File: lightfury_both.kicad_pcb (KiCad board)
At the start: 6 copper layers, 168.2 x 217.8 mm, 184 parts, among them U1 TLV61070ADBV, U1_2 TLV61070ADBV, U2 SN74LV1T126DBVR, U2_2 SN74LV1T126DBVR

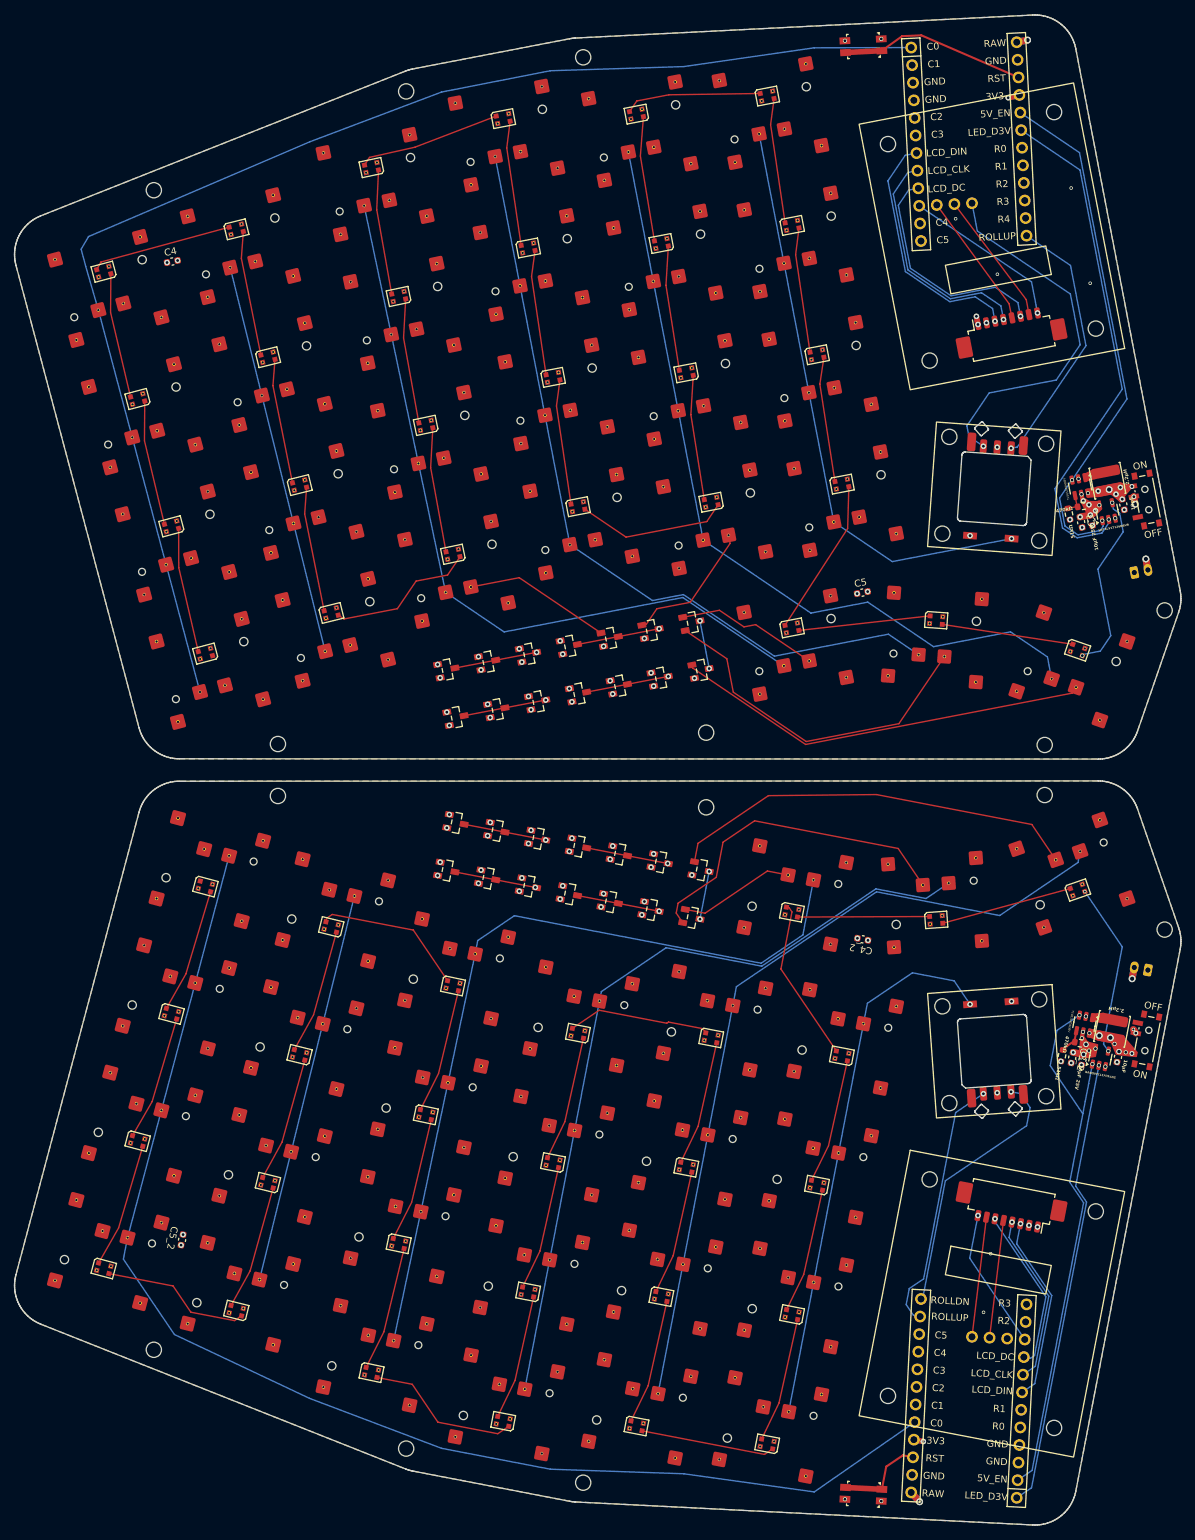
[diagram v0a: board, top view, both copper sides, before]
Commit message: Cleanup
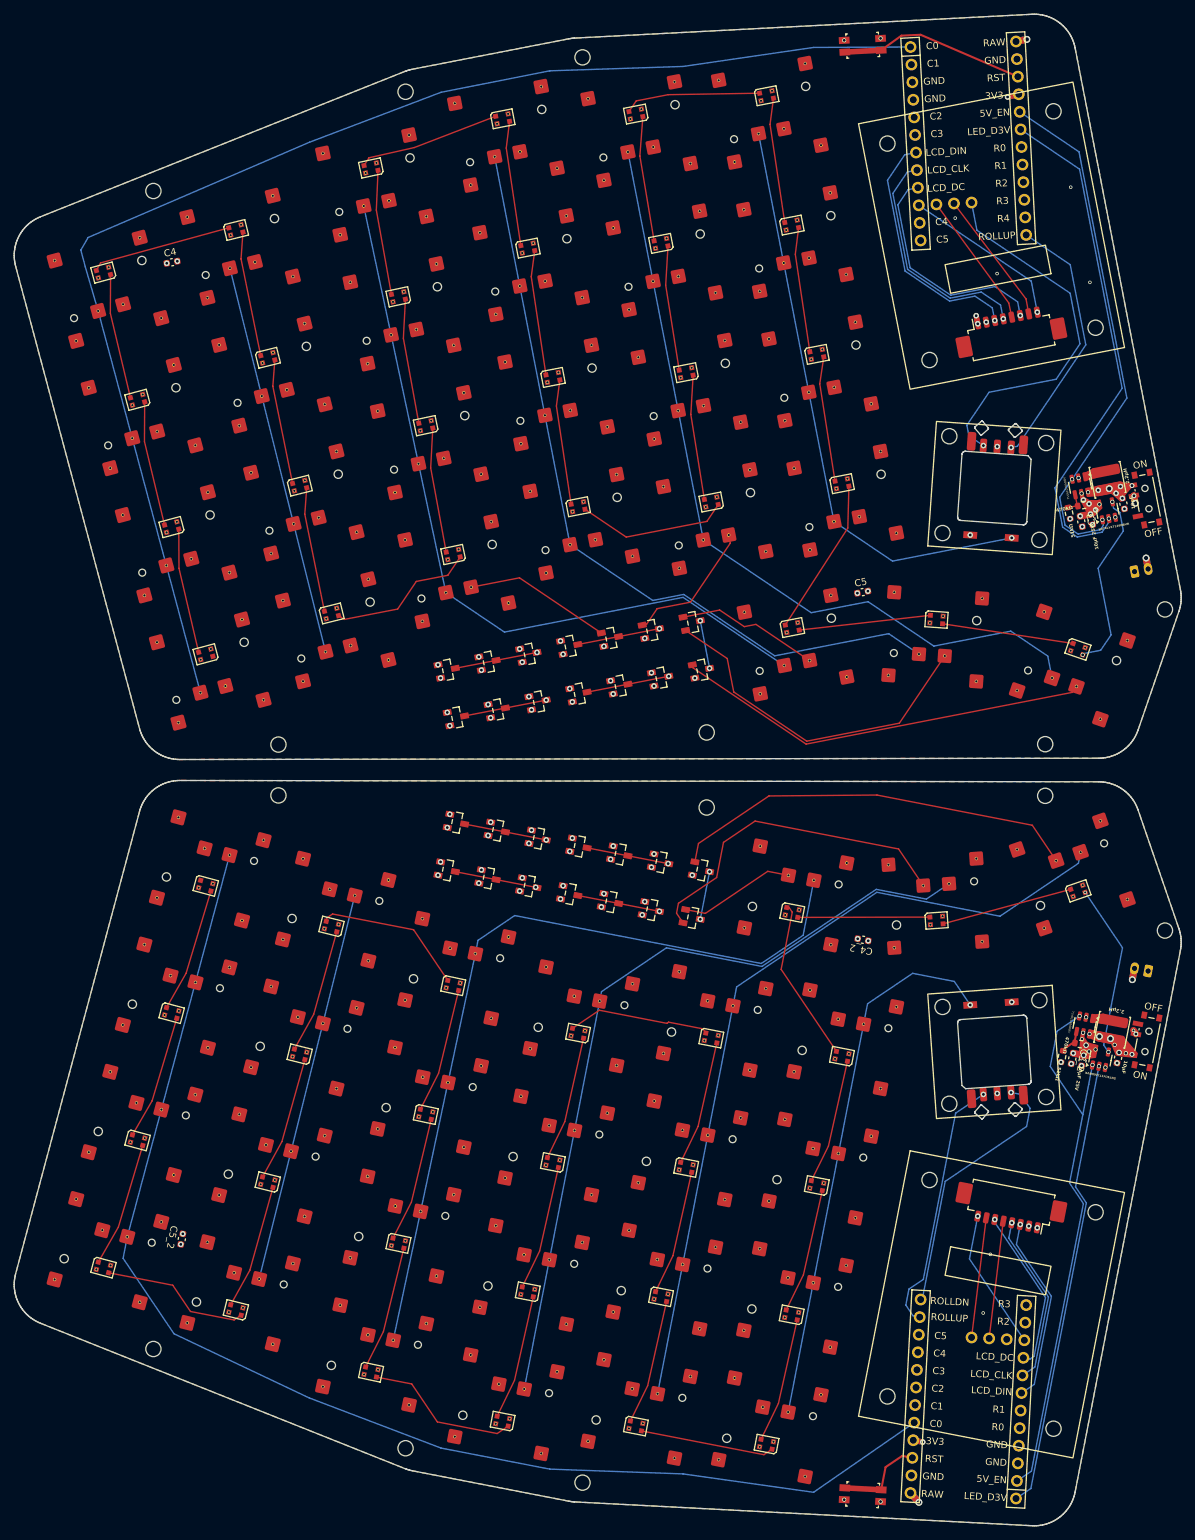
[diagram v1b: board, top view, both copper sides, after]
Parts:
- moved MH7_2 0.15 mm to (159.4, 128.4), turned to -161 degrees
- moved MH7 0.15 mm to (159.4, 82.0), turned to -19 degrees
- moved JST1 0.14 mm to (156.0, 76.4), turned to -169 degrees
- moved JST1_2 0.14 mm to (156.0, 134.0), turned to -11 degrees
- moved PWR1 0.14 mm to (156.8, 66.1), turned to 11 degrees
- moved PWR1_2 0.14 mm to (156.8, 144.3), turned to -11 degrees
- moved MH6_2 0.13 mm to (142.1, 108.9), turned to -161 degrees
- moved MH6 0.13 mm to (142.1, 101.5), turned to -19 degrees
- moved LED4 0.13 mm to (6.28, 33.5), turned to -165 degrees
- moved LED4_2 0.13 mm to (6.28, 176.9), turned to -15 degrees
- moved C1 0.13 mm to (153.4, 66.8), turned to -79 degrees
- moved S27_2 0.13 mm to (146.0, 120.3), turned to -161 degrees
- moved S27 0.13 mm to (146.0, 90.1), turned to -19 degrees
- moved LED27 0.13 mm to (146.8, 87.8), turned to -19 degrees
- moved LED15_2 0.13 mm to (146.8, 122.6), turned to 19 degrees
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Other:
- board size 168.2 x 217.8 mm -> 168.3 x 218 mm
